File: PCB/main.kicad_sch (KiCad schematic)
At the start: 1 part, among them U1 Raspberry_Pi_Pico

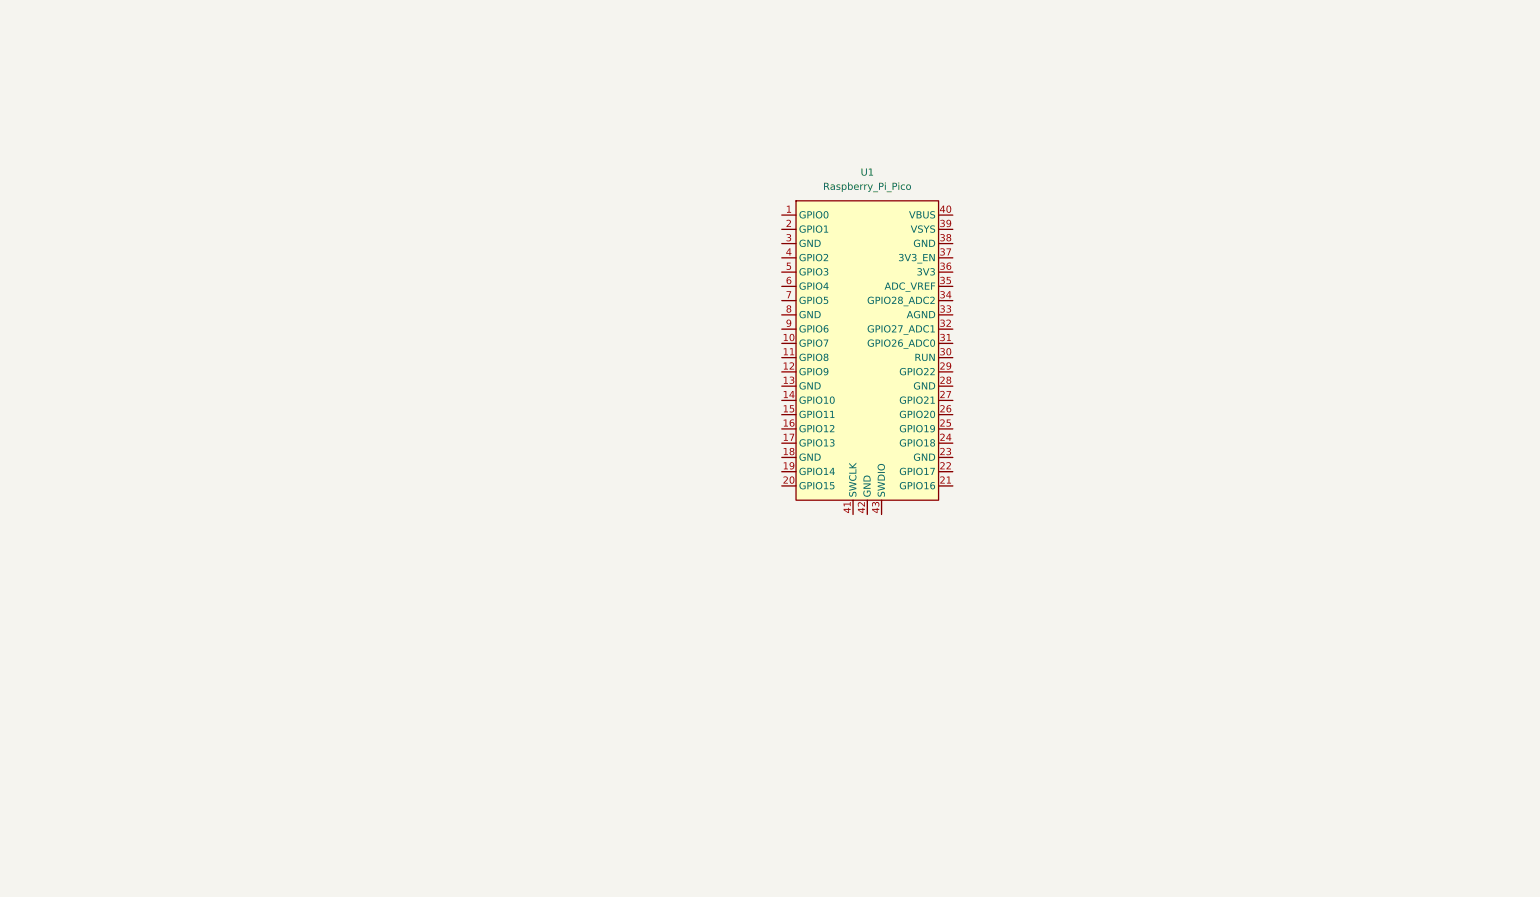
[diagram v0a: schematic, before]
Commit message: doin stuff
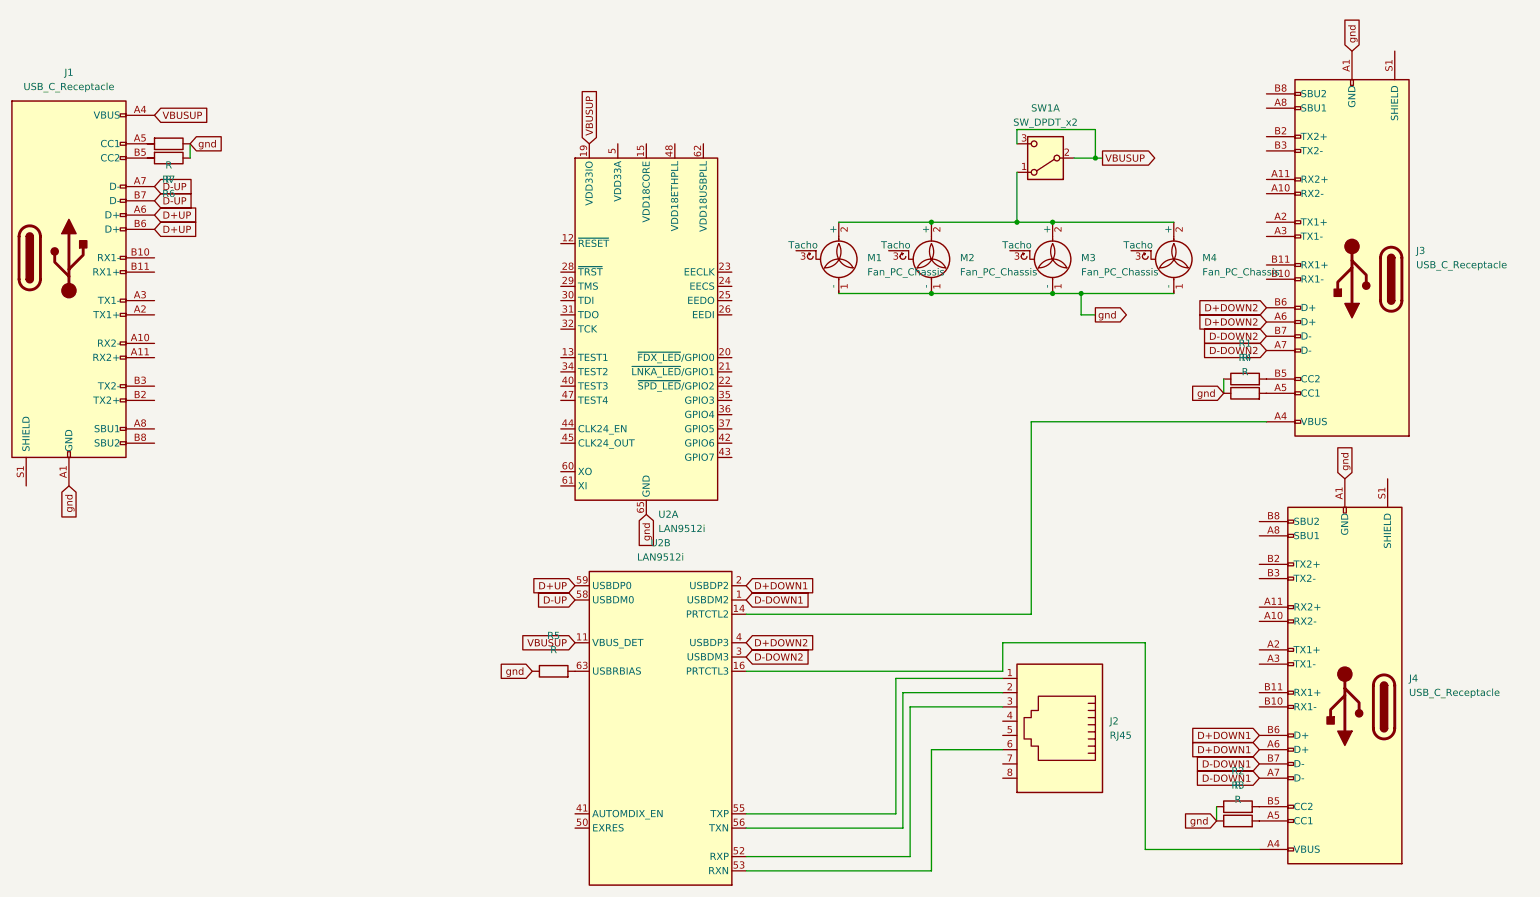
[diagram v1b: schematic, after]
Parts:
- removed U1: Raspberry_Pi_Pico, ScottoKeebs_MCU:Raspberry_Pi_Pico, symbol ScottoKeebs:MCU_Raspberry_Pi_Pico
- added J1, J3, J4: USB_C_Receptacle, Connector_USB:USB_C_Receptacle_Amphenol_12401548E4-2A_CircularHoles, symbol Connector:USB_C_Receptacle
- added J2: RJ45, Connector_RJ:RJ45_Amphenol_54602-x08_Horizontal, symbol Connector:RJ45
- added M1, M2, M3, M4: Fan_PC_Chassis, Connector:FanPinHeader_1x03_P2.54mm_Vertical, symbol Motor:Fan_PC_Chassis
- added R1, R2, R3, R4, R5, R6, R7: R, Resistor_SMD:R_0815_2038Metric, symbol Device:R
- added SW1: SW_DPDT_x2, Button_Switch_THT:SW_CK_JS202011CQN_DPDT_Straight, symbol Switch:SW_DPDT_x2
- added U2: LAN9512i, Package_DFN_QFN:QFN-64-1EP_9x9mm_P0.5mm_EP7.3x7.3mm, symbol Interface_Ethernet:LAN9512i
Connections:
- new net: U2.10 (VDD33A), U2.49 (VDD33A), U2.5 (VDD33A), U2.51 (VDD33A), U2.54 (VDD33A), U2.57 (VDD33A), U2.64 (VDD33A)
- new net: U2.15 (VDD18CORE), U2.38 (VDD18CORE)
- new net: J3.A4 (VBUS), J3.A9 (VBUS), J3.B4 (VBUS), J3.B9 (VBUS), U2.14 (PRTCTL2)
- new net: J4.A4 (VBUS), J4.A9 (VBUS), J4.B4 (VBUS), J4.B9 (VBUS), U2.16 (PRTCTL3)
- new net: J2.3, U2.52 (RXP)
- new net: J2.6, U2.53 (RXN)
- new net: J2.1, U2.55 (TXP)
- new net: J2.2, U2.56 (TXN)
- new net: R5.2, U2.63 (USBRBIAS)
- new net: M1.2 (+), M2.2 (+), M3.2 (+), M4.2 (+), SW1.1 (A)
- new net: J3.B5 (CC2), R1.2
- new net: J4.A5 (CC1), R3.2
- new net: J3.A5 (CC1), R4.2
- new net: J4.B5 (CC2), R2.2
- new net D+DOWN1: J4.A6 (D+), J4.B6 (D+), U2.2 (USBDP2)
- new net D+DOWN2: J3.A6 (D+), J3.B6 (D+), U2.4 (USBDP3)
- new net D+UP: J1.A6 (D+), J1.B6 (D+), U2.59 (USBDP0)
- new net D-DOWN1: J4.A7 (D-), J4.B7 (D-), U2.1 (USBDM2)
- new net D-DOWN2: J3.A7 (D-), J3.B7 (D-), U2.3 (USBDM3)
- new net D-UP: J1.A7 (D-), J1.B7 (D-), U2.58 (USBDM0)
- new net VBUSUP: J1.A4 (VBUS), J1.A9 (VBUS), J1.B4 (VBUS), J1.B9 (VBUS), SW1.2 (B), SW1.3 (C), U2.11 (VBUS_DET), U2.19 (VDD33IO), U2.27 (VDD33IO), U2.33 (VDD33IO), U2.39 (VDD33IO), U2.46 (VDD33IO)
- new net gnd: J1.A1 (GND), J1.A12 (GND), J1.B1 (GND), J1.B12 (GND), J3.A1 (GND), J3.A12 (GND), J3.B1 (GND), J3.B12 (GND), J4.A1 (GND), J4.A12 (GND), J4.B1 (GND), J4.B12 (GND), M1.1 (-), M2.1 (-), M3.1 (-), M4.1 (-), R1.1, R2.1, R3.1, R4.1, R5.1, R6.1, R7.1, U2.65 (GND)
